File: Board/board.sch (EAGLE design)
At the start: 49 parts, among them IC1 L297, IC2 MEGA32-P, IC3 L298, J1 +12V, Q1 BC639, Q3 BC639, U1 MCP9808MSOP, X1 WATER_PUMP, X2 FAN, X5 SM_CD, X6 SM_AB

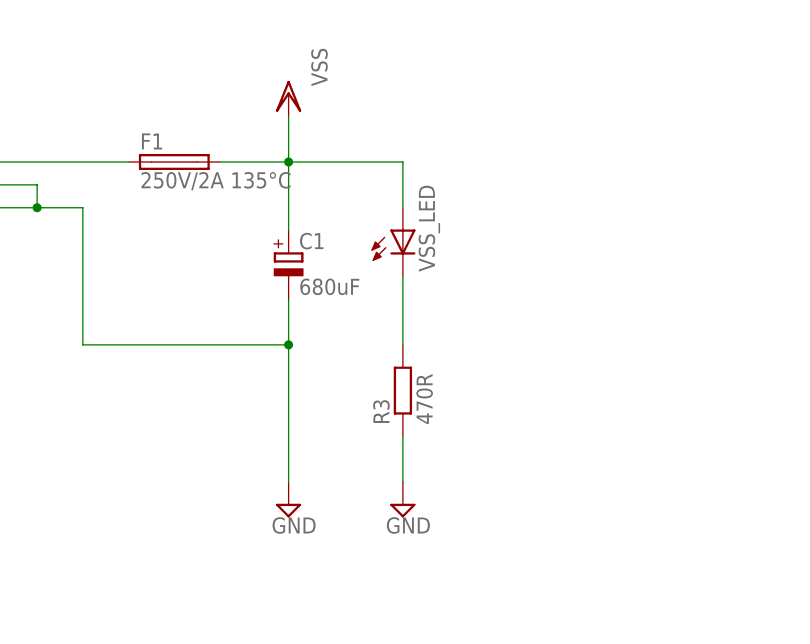
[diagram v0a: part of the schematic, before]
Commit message: auto route
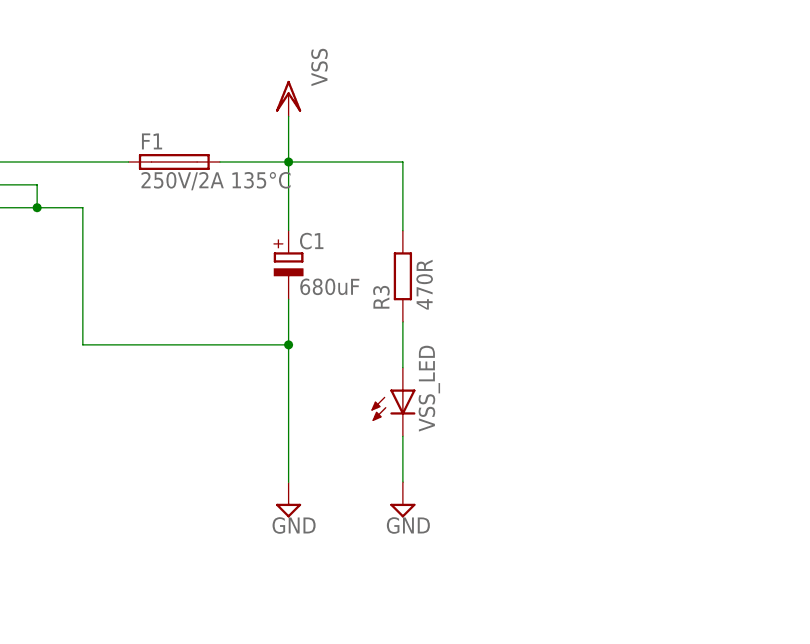
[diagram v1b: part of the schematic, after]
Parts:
- VSS_LED: device led:LED3MM -> led:LED5MM
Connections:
- net GND: now also VSS_LED.C; no longer R3.1
- net N$7: now also R3.1, VSS_LED.A; no longer R3.2, VSS_LED.C
- net VSS: now also R3.2; no longer VSS_LED.A
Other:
- moved on the sheet: R3, VSS_LED
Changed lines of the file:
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@@
 <part name="C11" library="rcl" deviceset="C-EU" device="025-025X050" value="100nF"/>
 <part name="SUPPLY29" library="supply2" deviceset="GND" device=""/>
-<part name="VSS_LED" library="led" deviceset="LED" device="3MM"/>
 <part name="R3" library="rcl" deviceset="R-EU_" device="0207/12" value="470R"/>
 <part name="SUPPLY30" library="supply2" deviceset="GND" device=""/>
@@
 <part name="FAN_LED" library="led" deviceset="LED" device="5MM"/>
 <part name="CTRL_LED" library="led" deviceset="LED" device="5MM"/>
+<part name="VSS_LED" library="led" deviceset="LED" device="5MM"/>
 </parts>
 <sheets>
@@
 <instance part="C11" gate="G$1" x="-73.66" y="-99.06"/>
 <instance part="SUPPLY29" gate="GND" x="-73.66" y="-109.22"/>
-<instance part="VSS_LED" gate="G$1" x="-45.72" y="134.62"/>
-<instance part="R3" gate="G$1" x="-45.72" y="116.84" rot="R90"/>
+<instance part="R3" gate="G$1" x="-45.72" y="129.54" rot="R90"/>
 <instance part="SUPPLY30" gate="GND" x="-45.72" y="104.14"/>
 <instance part="WP_LED" gate="G$1" x="457.2" y="-132.08"/>
 <instance part="FAN_LED" gate="G$1" x="457.2" y="-30.48"/>
 <instance part="CTRL_LED" gate="G$1" x="12.7" y="-27.94"/>
+<instance part="VSS_LED" gate="G$1" x="-45.72" y="116.84"/>
 </instances>
 <busses>
@@
 <junction x="-58.42" y="142.24"/>
 <wire x1="-58.42" y1="142.24" x2="-45.72" y2="142.24" width="0.1524" layer="91"/>
-<pinref part="VSS_LED" gate="G$1" pin="A"/>
-<wire x1="-45.72" y1="142.24" x2="-45.72" y2="137.16" width="0.1524" layer="91"/>
+<pinref part="R3" gate="G$1" pin="2"/>
+<wire x1="-45.72" y1="142.24" x2="-45.72" y2="134.62" width="0.1524" layer="91"/>
 </segment>
 <segment>
@@
 </segment>
 <segment>
-<pinref part="SUPPLY30" gate="GND" pin="GND"/>
-<pinref part="R3" gate="G$1" pin="1"/>
-<wire x1="-45.72" y1="106.68" x2="-45.72" y2="111.76" width="0.1524" layer="91"/>
-</segment>
-<segment>
 <pinref part="WP_LED" gate="G$1" pin="C"/>
 <pinref part="SUPPLY22" gate="GND" pin="GND"/>
@@
 <pinref part="SUPPLY25" gate="GND" pin="GND"/>
 <wire x1="12.7" y1="-33.02" x2="12.7" y2="-40.64" width="0.1524" layer="91"/>
+</segment>
+<segment>
+<pinref part="VSS_LED" gate="G$1" pin="C"/>
+<pinref part="SUPPLY30" gate="GND" pin="GND"/>
+<wire x1="-45.72" y1="111.76" x2="-45.72" y2="106.68" width="0.1524" layer="91"/>
 </segment>
 </net>
@@
 </segment>
 </net>
-<net name="N$7" class="0">
-<segment>
-<pinref part="R3" gate="G$1" pin="2"/>
-<pinref part="VSS_LED" gate="G$1" pin="C"/>
-<wire x1="-45.72" y1="121.92" x2="-45.72" y2="129.54" width="0.1524" layer="91"/>
-</segment>
-</net>
 <net name="N$11" class="0">
 <segment>
@@
 </segment>
 </net>
+<net name="N$7" class="0">
+<segment>
+<pinref part="R3" gate="G$1" pin="1"/>
+<pinref part="VSS_LED" gate="G$1" pin="A"/>
+<wire x1="-45.72" y1="124.46" x2="-45.72" y2="119.38" width="0.1524" layer="91"/>
+</segment>
+</net>
